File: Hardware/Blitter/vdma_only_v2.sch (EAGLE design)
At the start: 95 parts, among them IC1 74S08N, IC18 7432N, IC2 74ALS04N, IC20 7430N, IC21 7400N, IC31 7400N, IC32 7432N, IC5 74ALS00N, IC53 7404N, IC54 74LS07N, IC9 74LS74N, J1 TX25-40P-6ST-H1E, J2 TX25-40P-6ST-H1E

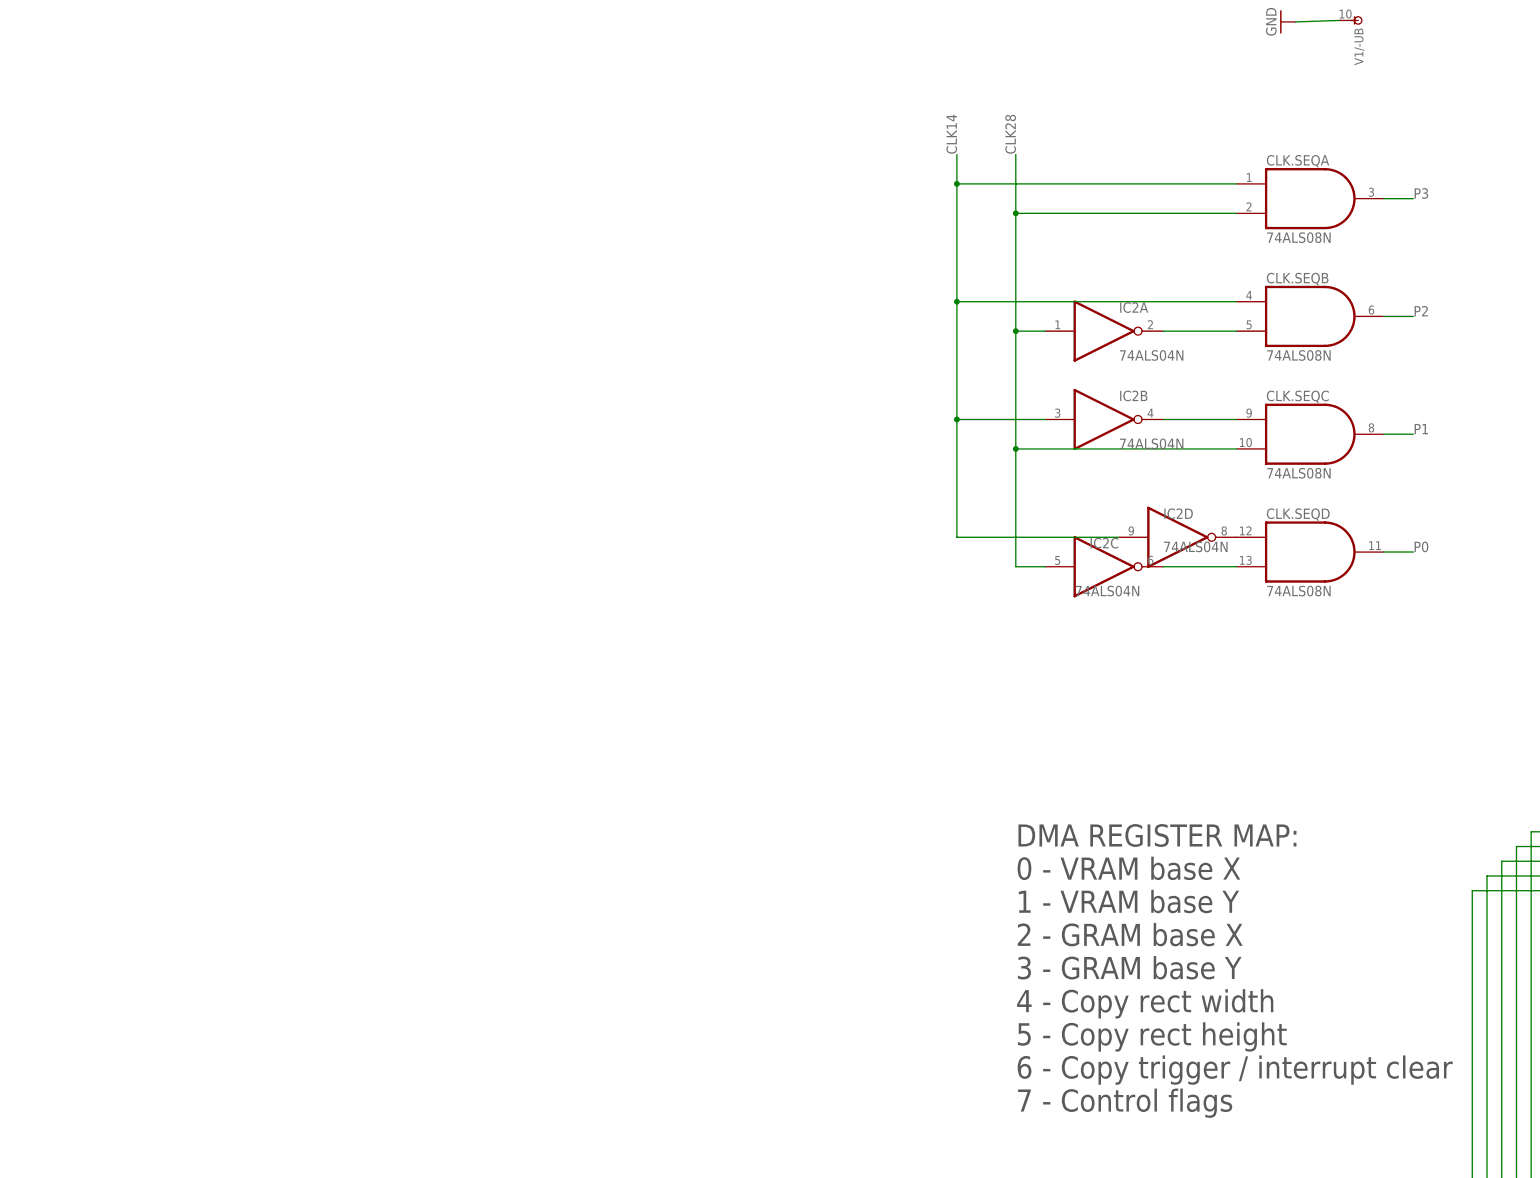
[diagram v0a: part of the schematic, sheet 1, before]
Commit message: Blitter fixes
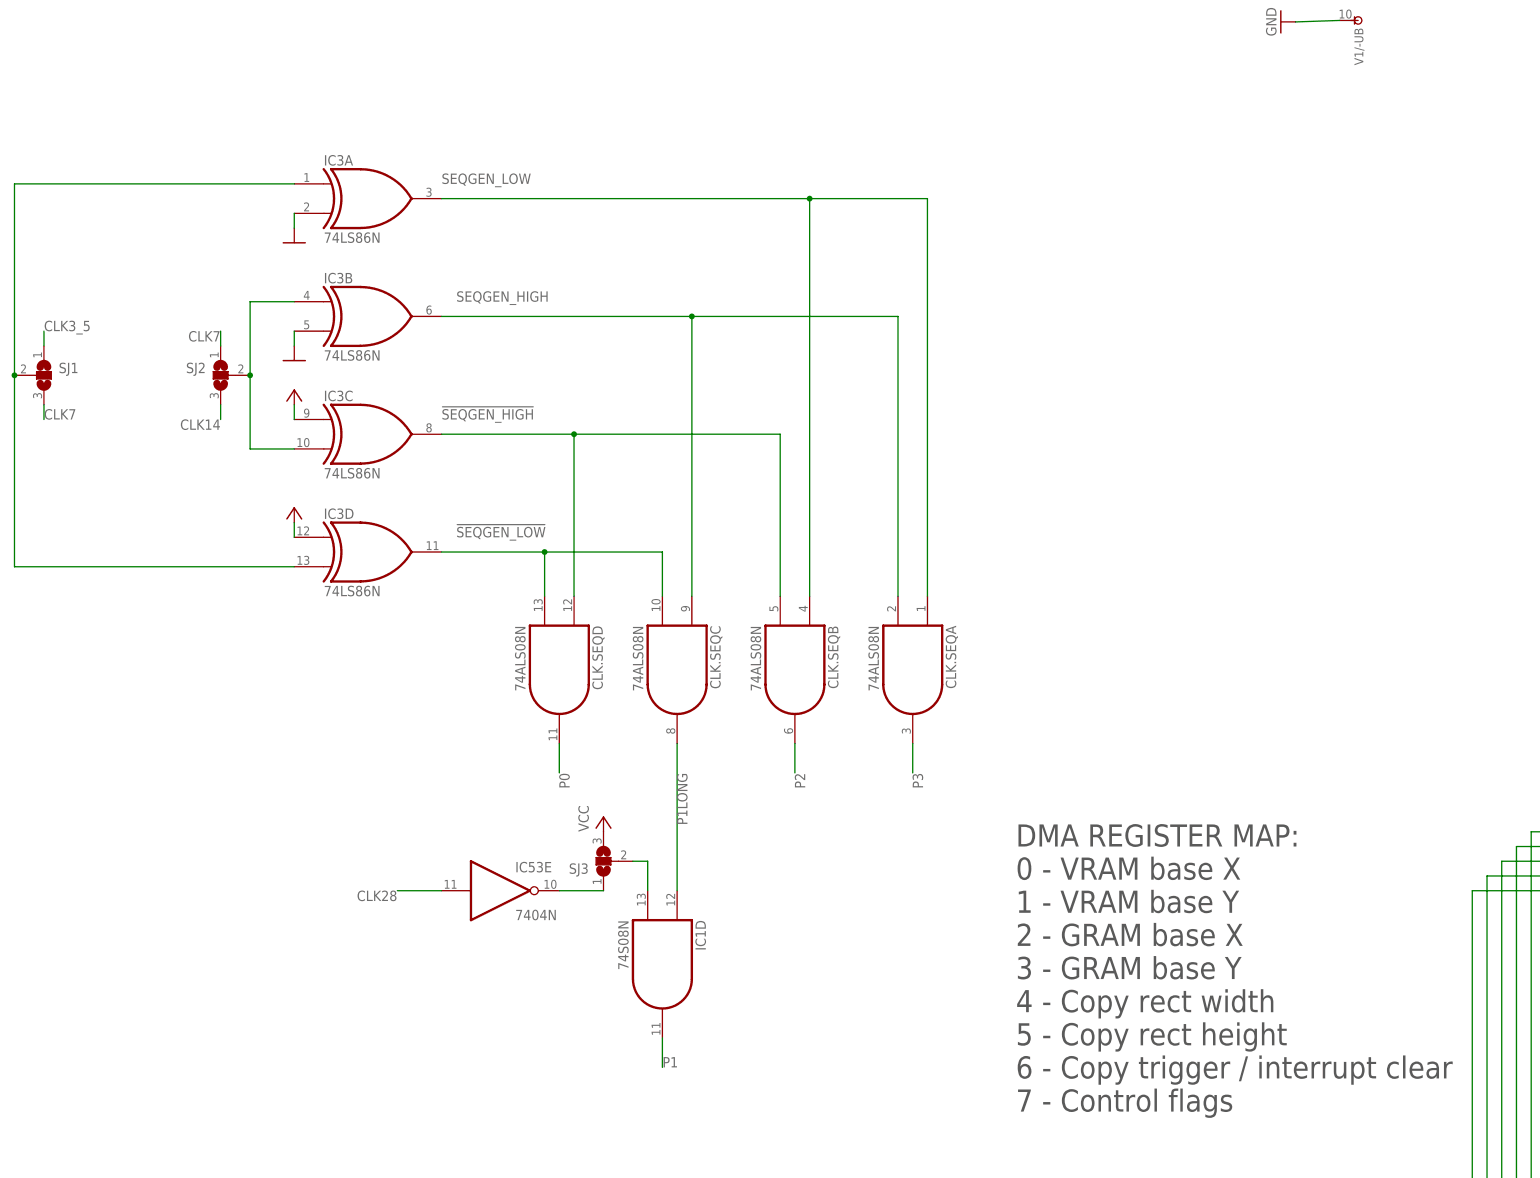
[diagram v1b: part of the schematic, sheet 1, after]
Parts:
- added IC3: 74LS86N, 74xx-us:74LS86N
- added SJ1, SJ2, SJ3: (no value), jumper:SJ2W
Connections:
- removed net N$86: CLK.SEQC.I0, IC2B.O
- new net !SEQGEN_HIGH: CLK.SEQB.I1, CLK.SEQD.I0, IC3C.O
- new net !SEQGEN_LOW: CLK.SEQC.I1, CLK.SEQD.I1, IC3D.O
- new net N$89: IC3A.I0, IC3D.I1, SJ1.2
- new net P1LONG: CLK.SEQC.O, IC1D.I0
- new net SEQGEN_HIGH: CLK.SEQA.I1, CLK.SEQC.I0, IC3B.O
- new net SEQGEN_LOW: CLK.SEQA.I0, CLK.SEQB.I0, IC3A.O
- net CLK14: now also SJ2.3; no longer CLK.SEQA.I0, CLK.SEQB.I0, IC2B.I, IC2D.I
- net CLK28: now also IC53E.I; no longer CLK.SEQA.I1, CLK.SEQC.I1, IC2A.I, IC2C.I
- net CLK3_5: now also SJ1.1
- net CLK7: now also SJ1.3, SJ2.1
- net GND: now also IC3A.I1, IC3B.I1
- net N$83: now also IC3B.I0, IC3C.I1, SJ2.2; no longer CLK.SEQD.I1, IC2C.O
- net N$84: now also IC53E.O, SJ3.1; no longer CLK.SEQD.I0, IC2D.O
- net N$85: now also IC1D.I1, SJ3.2; no longer CLK.SEQB.I1, IC2A.O
- net P1: now also IC1D.O; no longer CLK.SEQC.O
- net VCC: now also IC3C.I0, IC3D.I0, SJ3.3
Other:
- moved on the sheet: CLK.SEQA, CLK.SEQB, CLK.SEQC, CLK.SEQD
